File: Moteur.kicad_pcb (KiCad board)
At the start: 4 copper layers, 31.7 x 16.1 mm, 53 parts, among them IC1 TPS71501, IC2 TLV710, IC3 MAX3051, IC4 LM5106, IC5 LM5106, IC6 INA282, P1 Bus2, P2 MOTOR, P3 GPIO, P4 CONN_1, P5 DBG, P6 CONN_1, Q1 IRF8721, Q2 IRF8721, Q3 IRF8721, Q4 IRF8721, U1 STM32F303CCT6, X1 16MHz

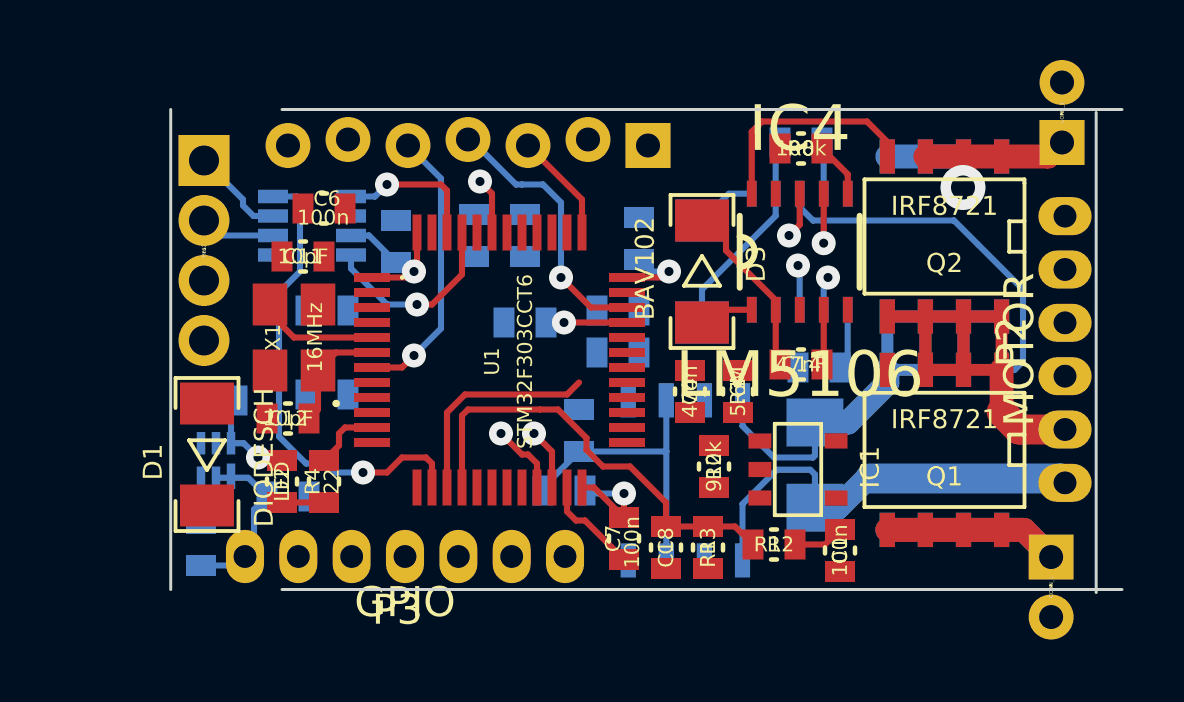
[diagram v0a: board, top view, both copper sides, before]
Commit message: routing
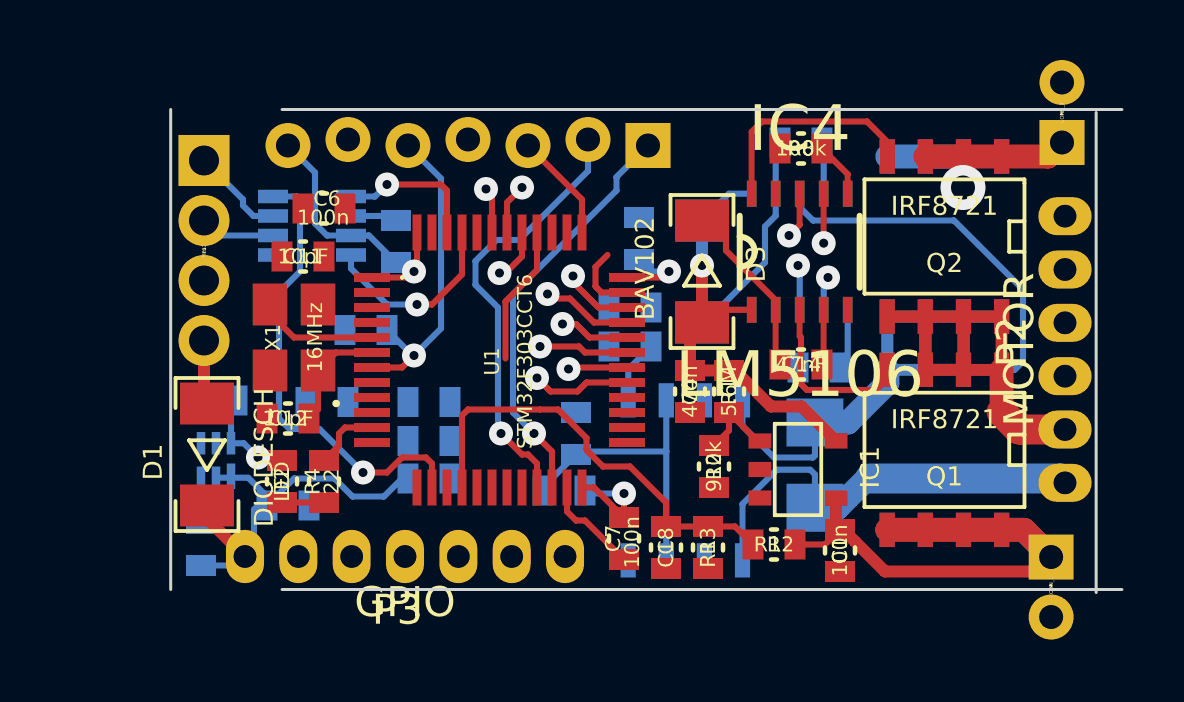
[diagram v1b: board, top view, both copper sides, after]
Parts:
- moved R5 7.01 mm to (130.9, 101.0), turned to 0 degrees
- moved R3 6.41 mm to (130.9, 99.8), turned to 0 degrees
- moved R6 6.11 mm to (130.9, 102.3)
- moved C5 1.45 mm to (128.8, 97.3)
- moved R9 0.45 mm to (137.6, 97.9)
- moved C15 0.41 mm to (137.6, 96.6)
- moved C17 0.30 mm to (126.2, 103.2)
- moved R1 0.30 mm to (140.9, 99.4)
- moved C10 0.25 mm to (127.5, 99.8)
- moved C8 0.14 mm to (135.8, 100.8)
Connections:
- IC4 pad 7: Mot_En_1 -> Mot_En_2
- IC4 pad 8: PWM1 -> PWM2
- IC5 pad 7: Mot_En_2 -> Mot_En_1
- IC5 pad 8: PWM2 -> PWM1
- P3 pad 1: GPIO_ADC -> I
- P3 pad 2: I -> GPIO_B
- P3 pad 3: GPIO_B -> GPIO_A
- P3 pad 4: GPIO_A -> GPIO_ADC
- P3 pad 5: GND -> +3.3V_A
- P3 pad 6: +3.3V_A -> GND
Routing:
- net +5V_protected: track 5.97 -> 31.2 mm
- net B: track 1.87 -> 22.7 mm
- net A: track 0.00 -> 20.8 mm, vias 0 -> 1
- net Mot_En_1: track 1.71 -> 18.3 mm, vias 1 -> 2
- net PWM1: track 1.54 -> 15.4 mm, vias 1 -> 2
- net Mot_En_2: track 1.14 -> 15.0 mm, vias 1 -> 2
- net Tx: track 2.41 -> 14.6 mm
- net Rx: track 2.05 -> 13.8 mm
- net PWM2: track 1.50 -> 12.7 mm, vias 1 -> 2
- net +9V: track 3.86 -> 14.9 mm, vias 0 -> 1
- net +BATT: track 13.4 -> 22.3 mm
- net ADC/I_MOT: track 7.31 -> 0.00 mm
- net Swdio: track 9.08 -> 2.35 mm
- net N-0000043: track 0.00 -> 5.90 mm
- net GPIO_A: track 0.00 -> 4.63 mm
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
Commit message: routing
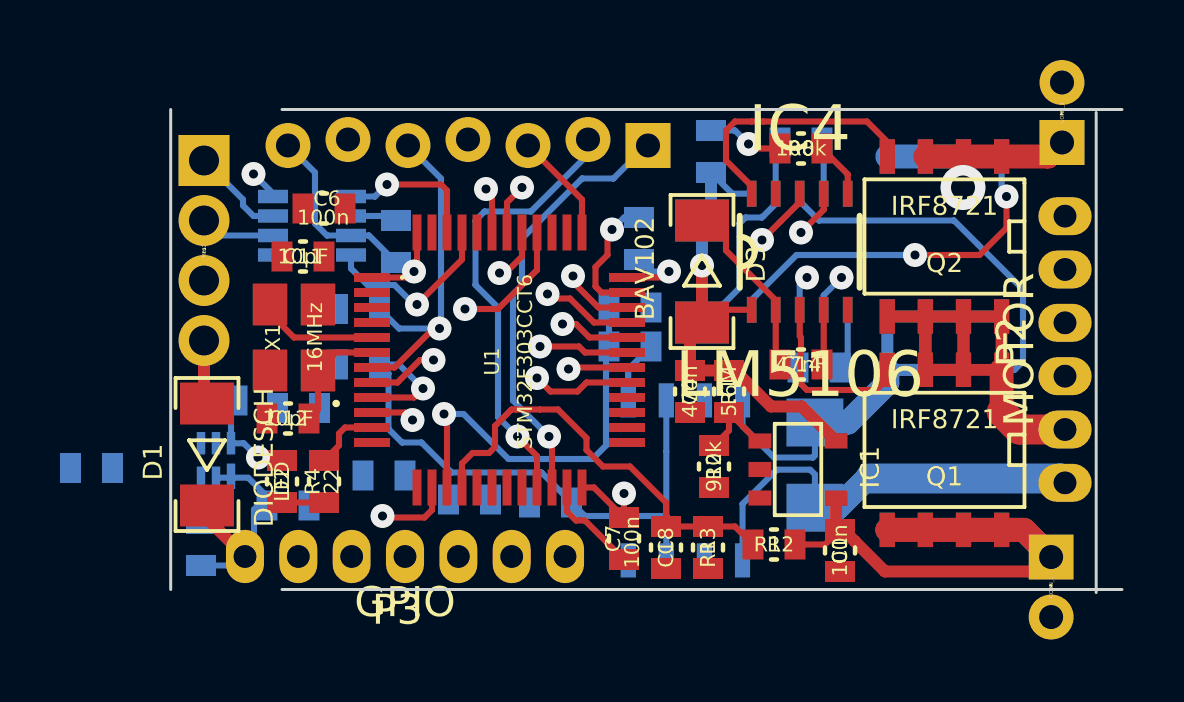
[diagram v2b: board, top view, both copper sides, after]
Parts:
- added C19: 100nF (DNP), _0603, B.Cu at (140.3, 91.4)
- moved R3 11.5 mm to (119.7, 102.0)
- moved L1 9.27 mm to (126.5, 100.0), turned to 0 degrees
- moved C8 2.45 mm to (134.9, 103.1), turned to 180 degrees
- moved R5 1.89 mm to (129.4, 102.2)
- moved C10 1.63 mm to (128.6, 98.5)
- moved R6 1.52 mm to (132.2, 103.0)
- moved C5 0.74 mm to (128.6, 96.7)
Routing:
- net +5V_protected: track 31.2 -> 8.20 mm
- net ADC/I_MOT: track 0.00 -> 13.3 mm, vias 0 -> 1
- net N-0000040: track 0.00 -> 12.3 mm, vias 0 -> 2
- net +3.3V_A: track 10.0 -> 21.7 mm, vias 0 -> 1
- net I: track 3.04 -> 13.5 mm
- net GPIO_B: track 1.78 -> 11.9 mm
- net GPIO_A: track 4.63 -> 12.6 mm, vias 0 -> 1
- net GND: track 16.6 -> 23.5 mm, vias 1 -> 4
- net Swdio: track 2.35 -> 9.12 mm
- net GPIO_ADC: track 0.00 -> 6.11 mm, vias 0 -> 1
- net CAN_SPEED: track 15.5 -> 17.3 mm, vias 1 -> 2
- net +9V: track 14.9 -> 16.6 mm
- net +3.3V: track 19.8 -> 18.5 mm
- net N-0000038: track 7.50 -> 8.73 mm
- net Reset: track 10.6 -> 11.7 mm
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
